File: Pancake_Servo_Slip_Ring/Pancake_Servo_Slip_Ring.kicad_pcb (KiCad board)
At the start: 2 copper layers, 67 x 67 mm, 1 part

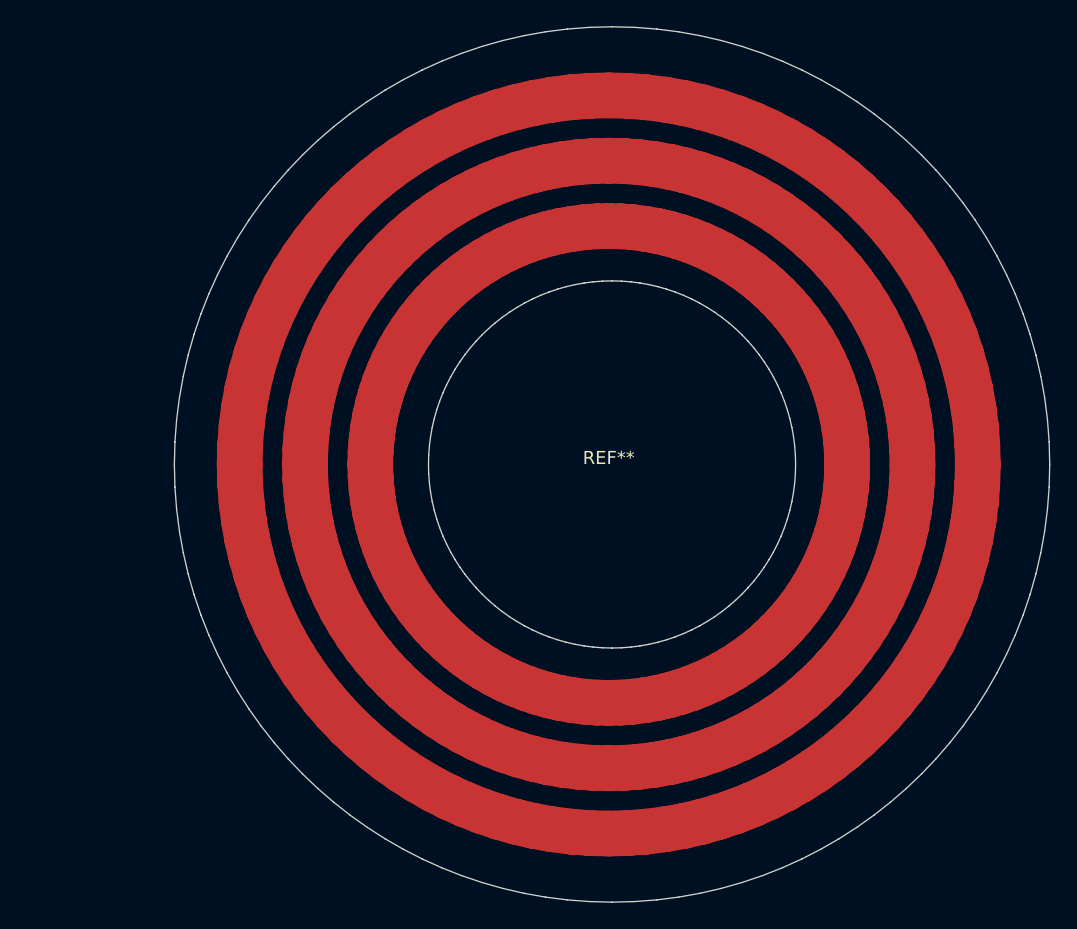
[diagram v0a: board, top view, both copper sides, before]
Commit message: Updated C3P0 Controller
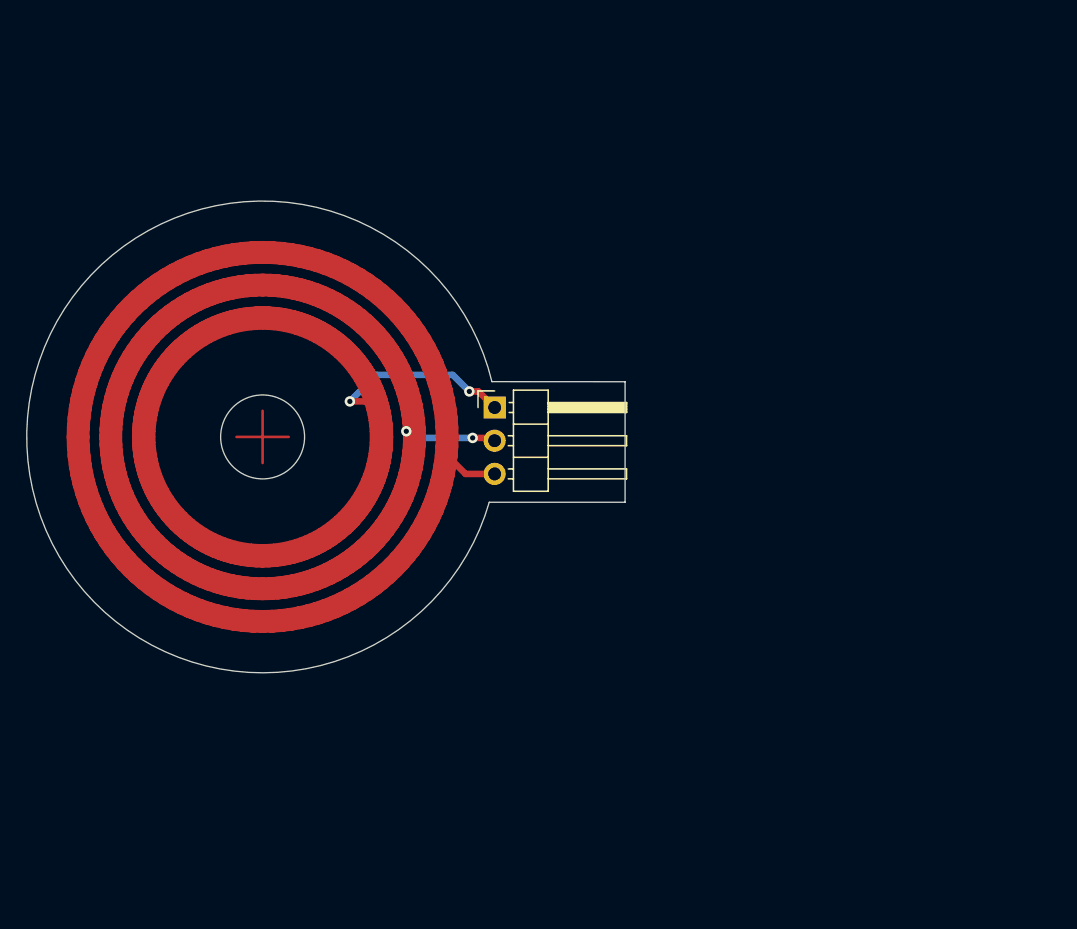
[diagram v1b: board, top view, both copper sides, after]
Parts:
- removed the REF** at (126.5, 102.1)
- added REF**: PinHeader_1x03_P2.54mm_Horizontal, Connector_PinHeader_2.54mm:PinHeader_1x03_P2.54mm_Horizontal, F.Cu at (117.8, 97.8)
- added REF**: Slip_Ring_V2, Logos:Slip_Ring_V2, F.Cu at (100.0, 100.0)
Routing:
- net (no net): track 0.00 -> 30.6 mm, vias 0 -> 4
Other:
- board size 67 x 67 mm -> 45.8 x 36.1 mm
